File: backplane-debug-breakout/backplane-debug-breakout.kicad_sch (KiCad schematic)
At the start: 11 parts, among them J1 Conn_02x08_Odd_Even, J2 Conn_01x04, J3 Conn_01x01_Socket, J4 Conn_01x01_Socket, J5 Conn_01x04, SW2 SW_Omron_B3FS, SW3 EG1218, U1 UMFT234XF

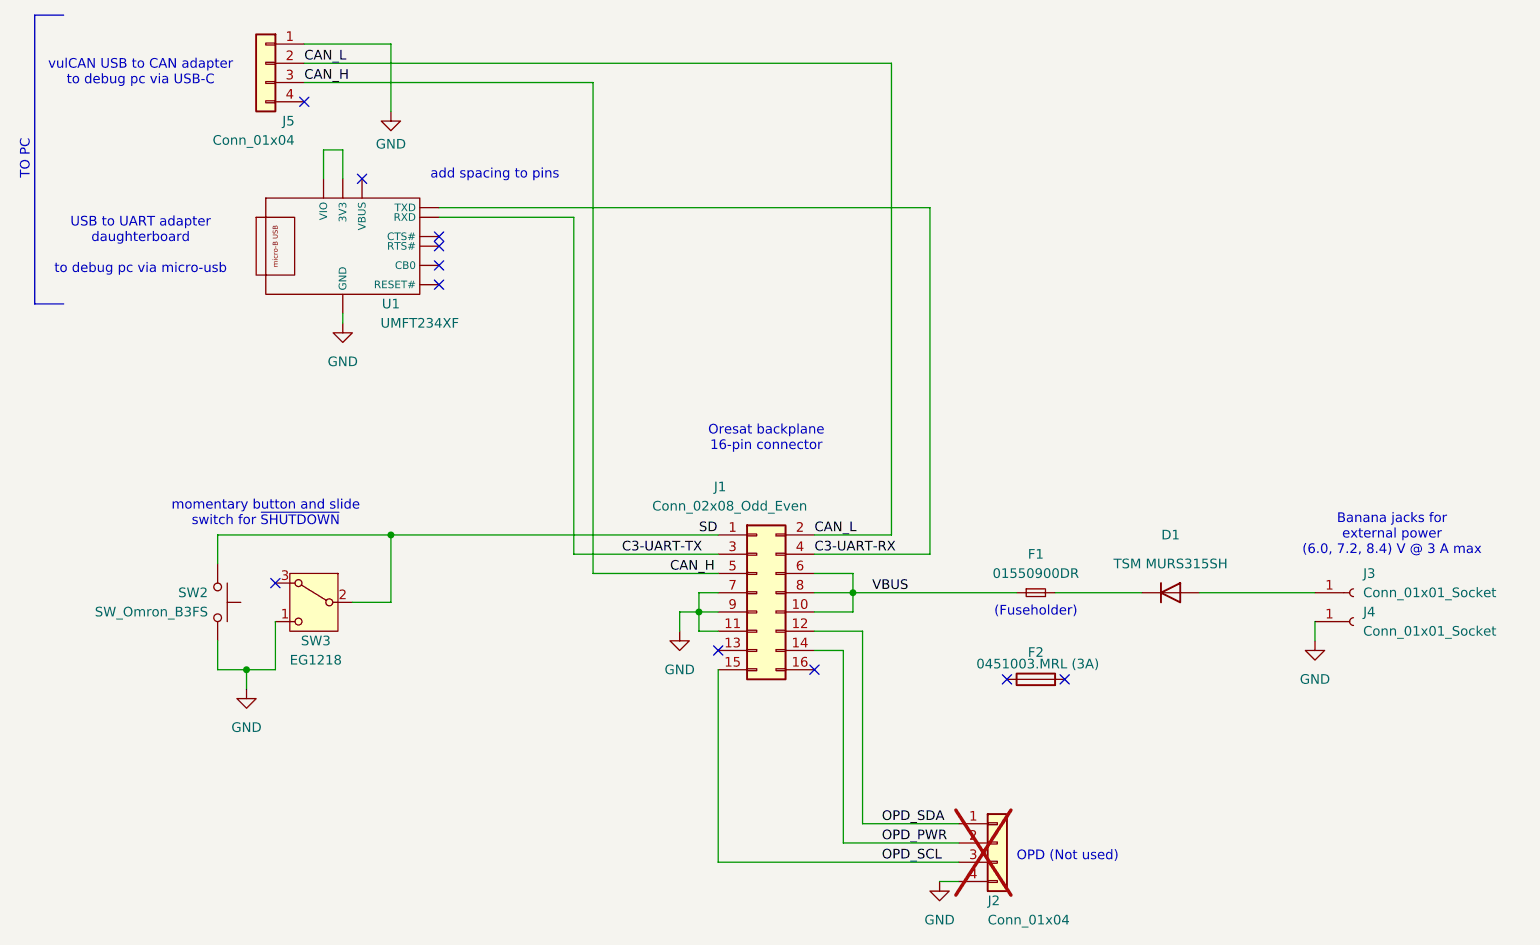
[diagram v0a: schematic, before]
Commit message: updated schematic
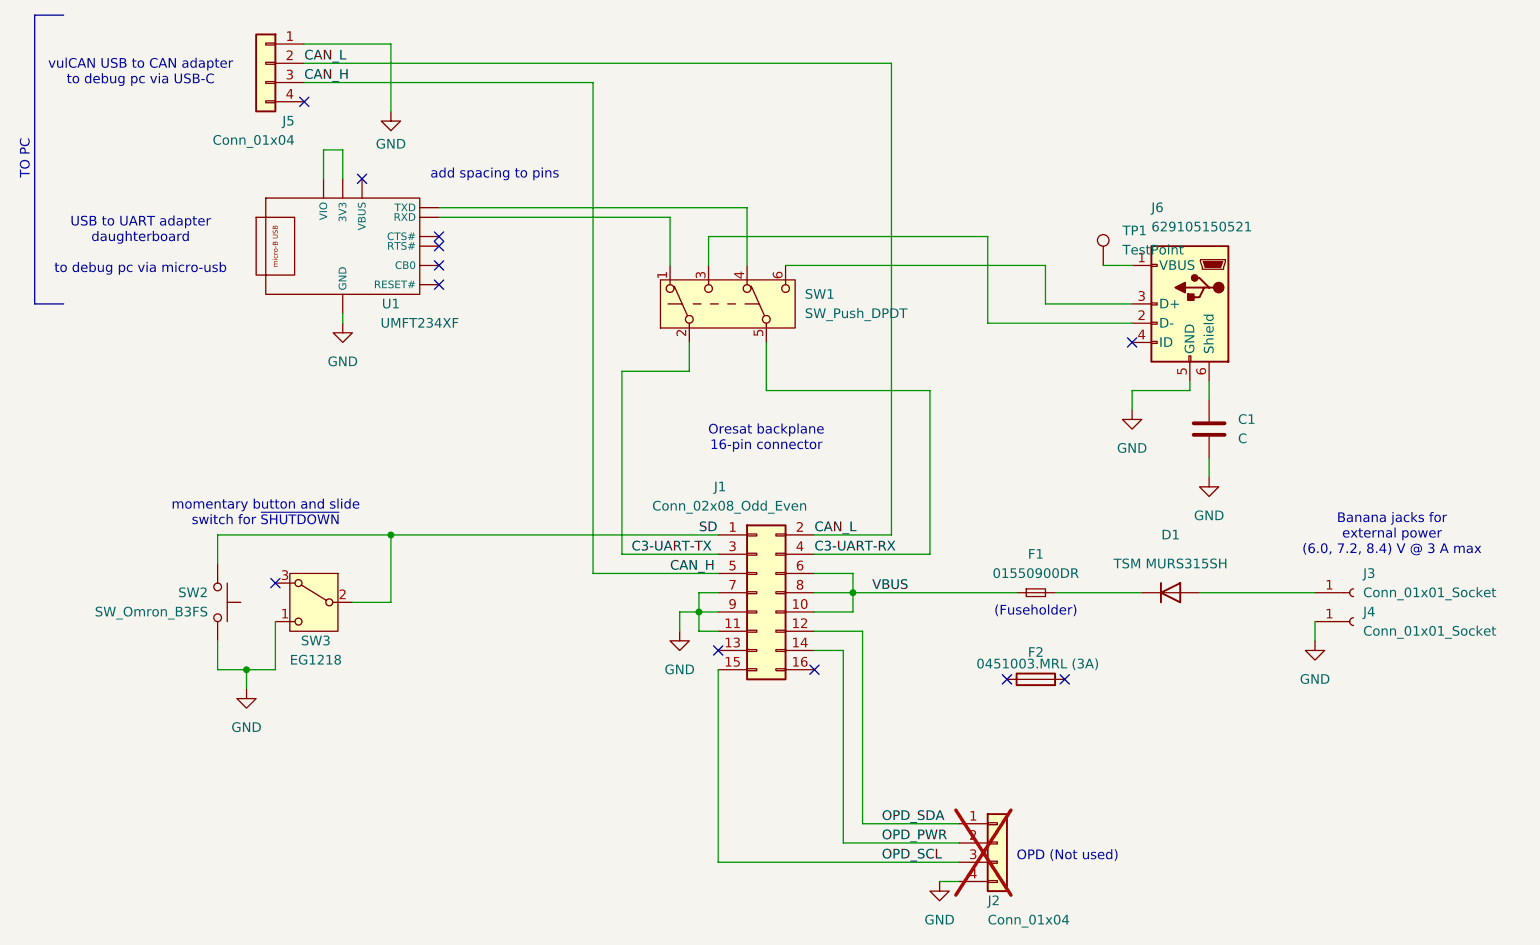
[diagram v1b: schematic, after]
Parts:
- added C1: C, symbol Device:C
- added J6: 629105150521, Connector_USB:USB_Micro-B_Wuerth_629105150521_CircularHoles, symbol Connector:USB_B_Micro
- added SW1: SW_Push_DPDT, symbol Switch:SW_Push_DPDT
- added TP1: TestPoint, symbol Connector:TestPoint
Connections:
- net C3-UART-RX: now also SW1.5 (B); no longer U1.P7 (TXD)
- net C3-UART-TX: now also SW1.2 (B); no longer U1.P9 (RXD)
- net GND: now also C1.2, J6.5 (GND)
- new net: SW1.1 (A), U1.P9 (RXD)
- new net: J6.2 (D-), SW1.3 (C)
- new net: SW1.4 (A), U1.P7 (TXD)
- new net: J6.3 (D+), SW1.6 (C)
- new net: C1.1, J6.6 (Shield)
- new net: J6.1 (VBUS), TP1.1
- no-connect marks 11 -> 12
